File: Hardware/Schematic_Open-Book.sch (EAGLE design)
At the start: 103 parts, among them IC1 BD5229G-TR, IC4 XC6220A331MR-G, J1 FH34SRJ-24S-0.5SH_99_, J2 SAMACSYS_PARTS_USB4110-GF-A, J3 QWIIC_RIGHT_ANGLE, J4 112A-TAAR-R03_ATTEND, Q1 20V/4.2A/52mΩ/1.4W, Q2 20V/4.2A/52mΩ/1.4W, Q3 SI1308EDL-T1-GE3, U1 W25Q512JVEIQ, U2 ESP32-C6-WROOM-1-N8, U3 DS3231SN#, U4 MAX17048G+T10

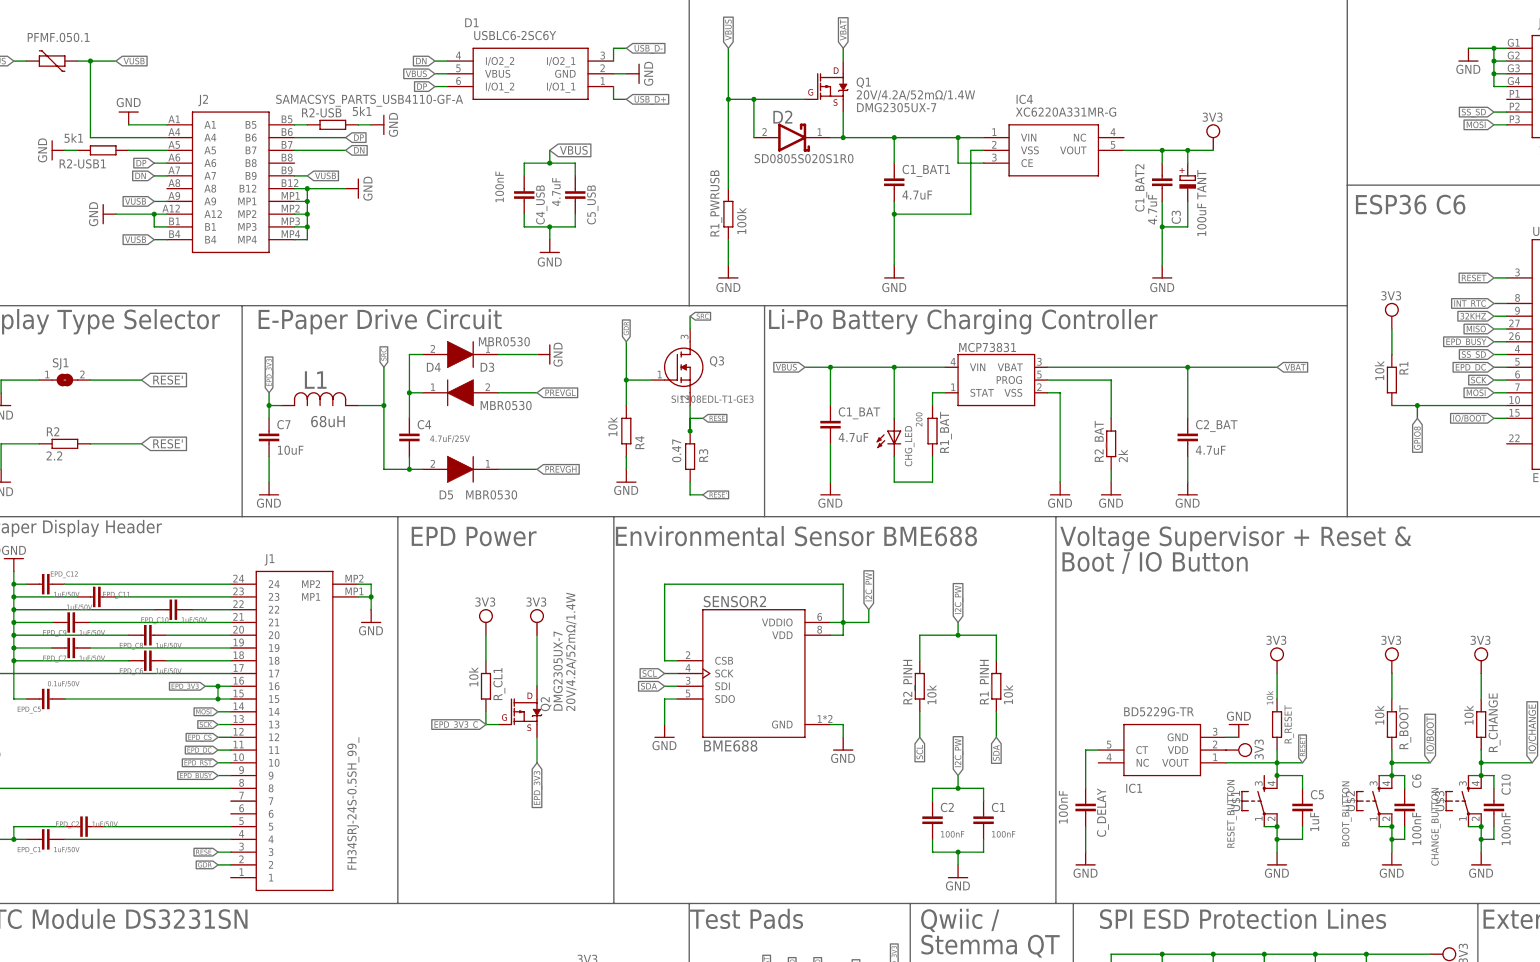
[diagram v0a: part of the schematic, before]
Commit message: update
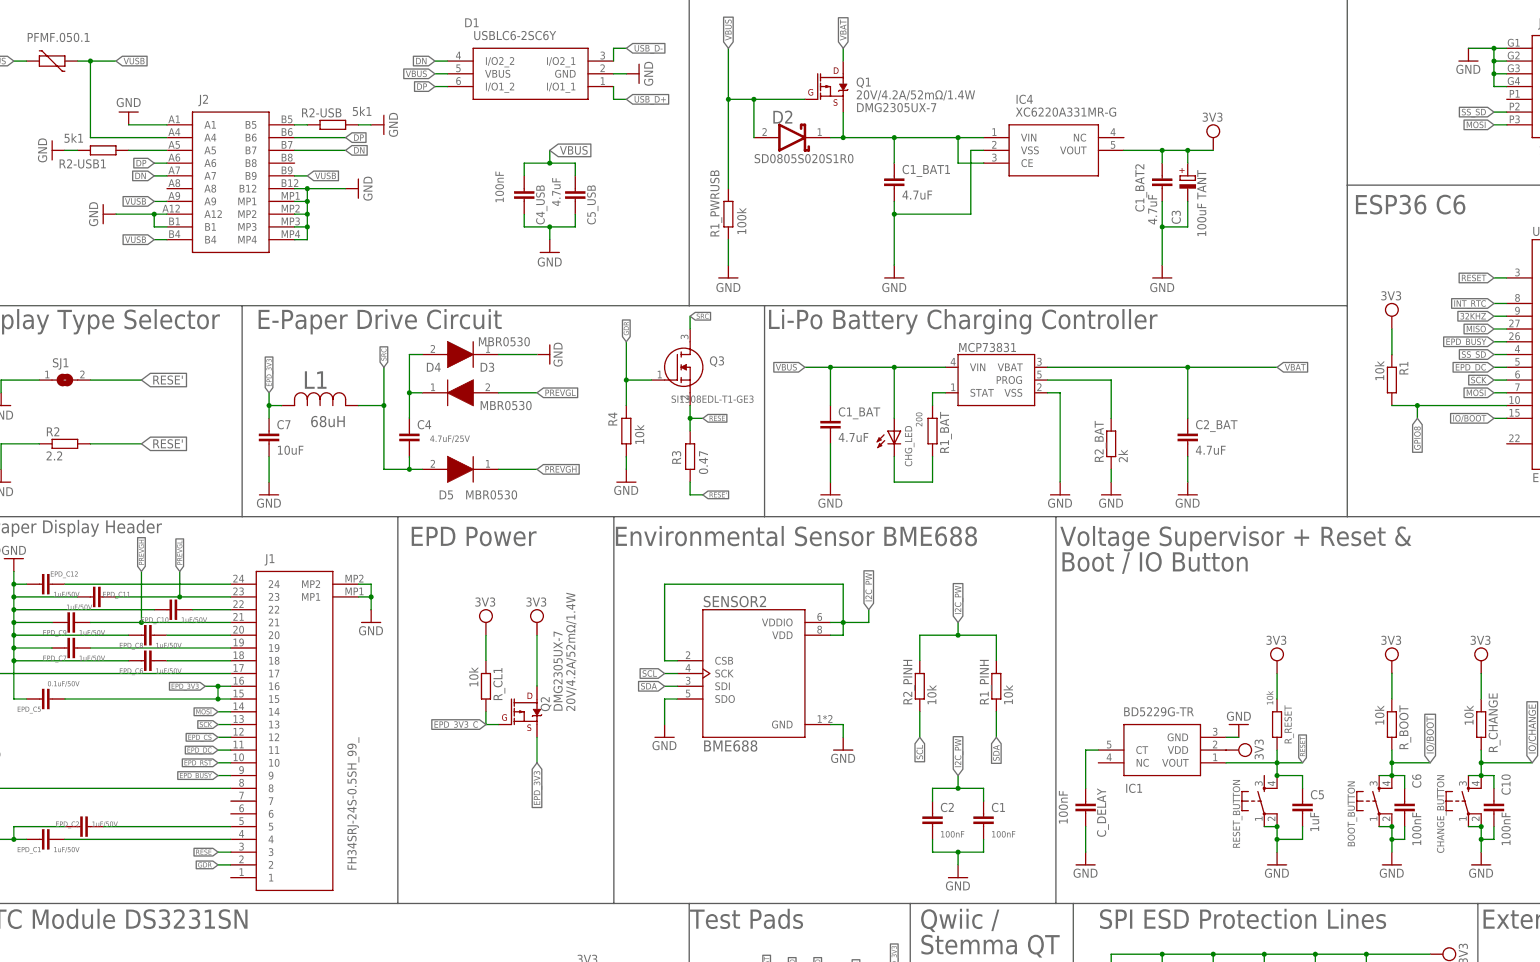
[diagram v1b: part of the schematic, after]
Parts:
- renumbered U$1 to RESET_BUTTON, U$2 to BOOT_BUTTON, U$3 to CHANGE_BUTTON
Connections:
- removed net N$21: EPD_C11.1, J1.23
- removed net N$25: EPD_C9.1, J1.21
- net GDR: now also R4.1; no longer R4.2
- net GND: now also R4.2; no longer R4.1
- net PREVGH: now also EPD_C9.1, J1.21
- net PREVGL: now also EPD_C11.1, J1.23
- net RESE: now also R3.1; no longer R3.2
- net RESE': now also R3.2; no longer R3.1
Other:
- moved on the sheet: R3, R4
